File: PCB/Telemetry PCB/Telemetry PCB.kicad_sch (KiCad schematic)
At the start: 40 parts, among them IC1 E22-900M22S, J1 Conn_01x04_Pin, J2 GPS, J3 Batt, J4 Serial Debug Header 1x4, SW1 SW_MEC_5E, SW2 SW_MEC_5E, U1 STM32F411CEUx, U2 AP62200WU, U3 MCP1700x-250xxTT, Y1 25MHZ 9pF, Y2 32.768k 6pF

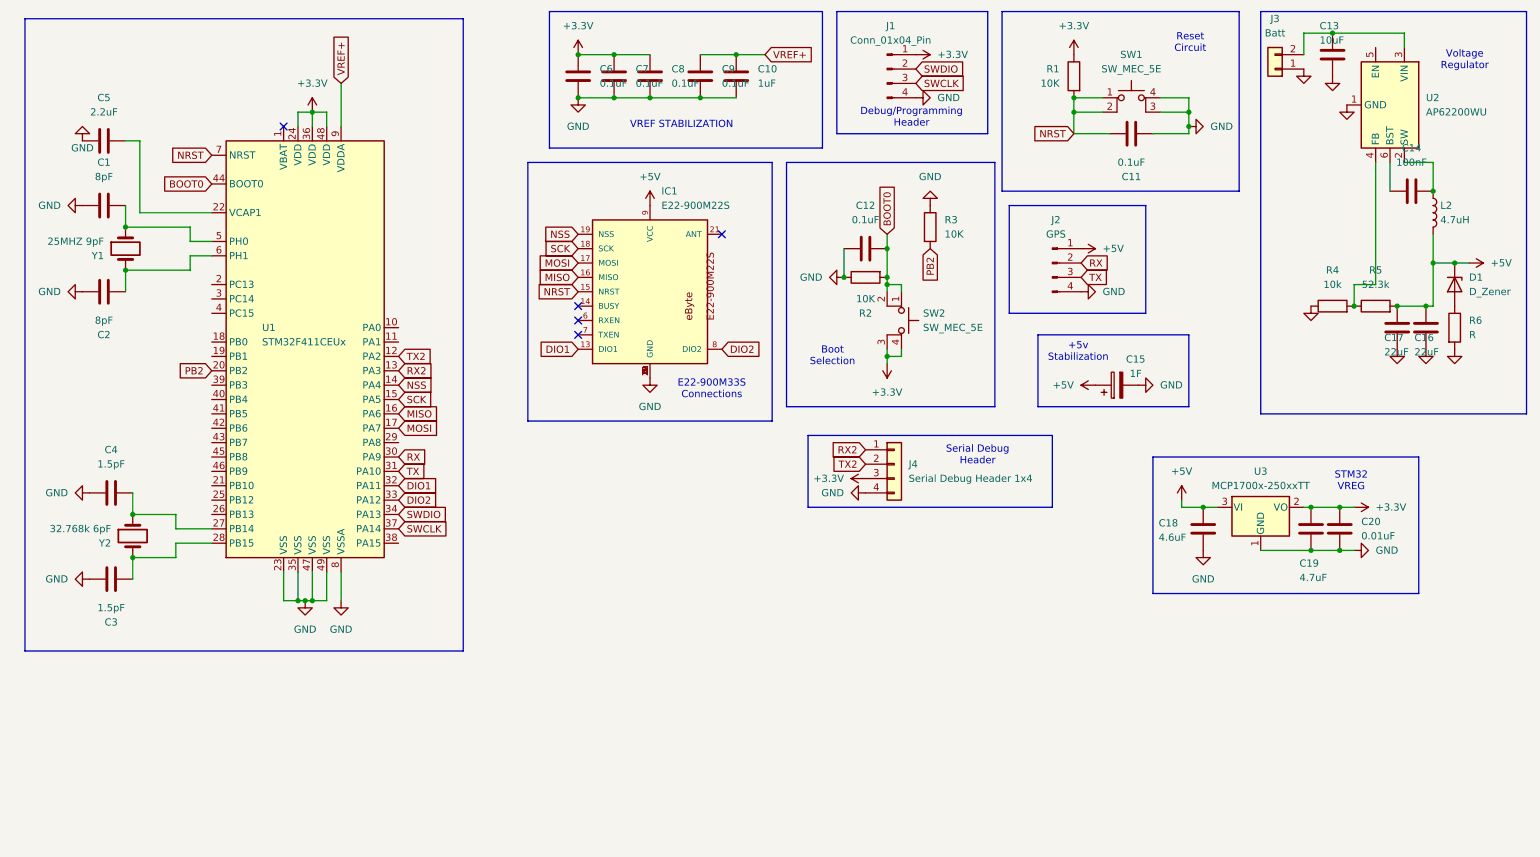
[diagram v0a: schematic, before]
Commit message: see last push discription
Last push did not work. see last push for description
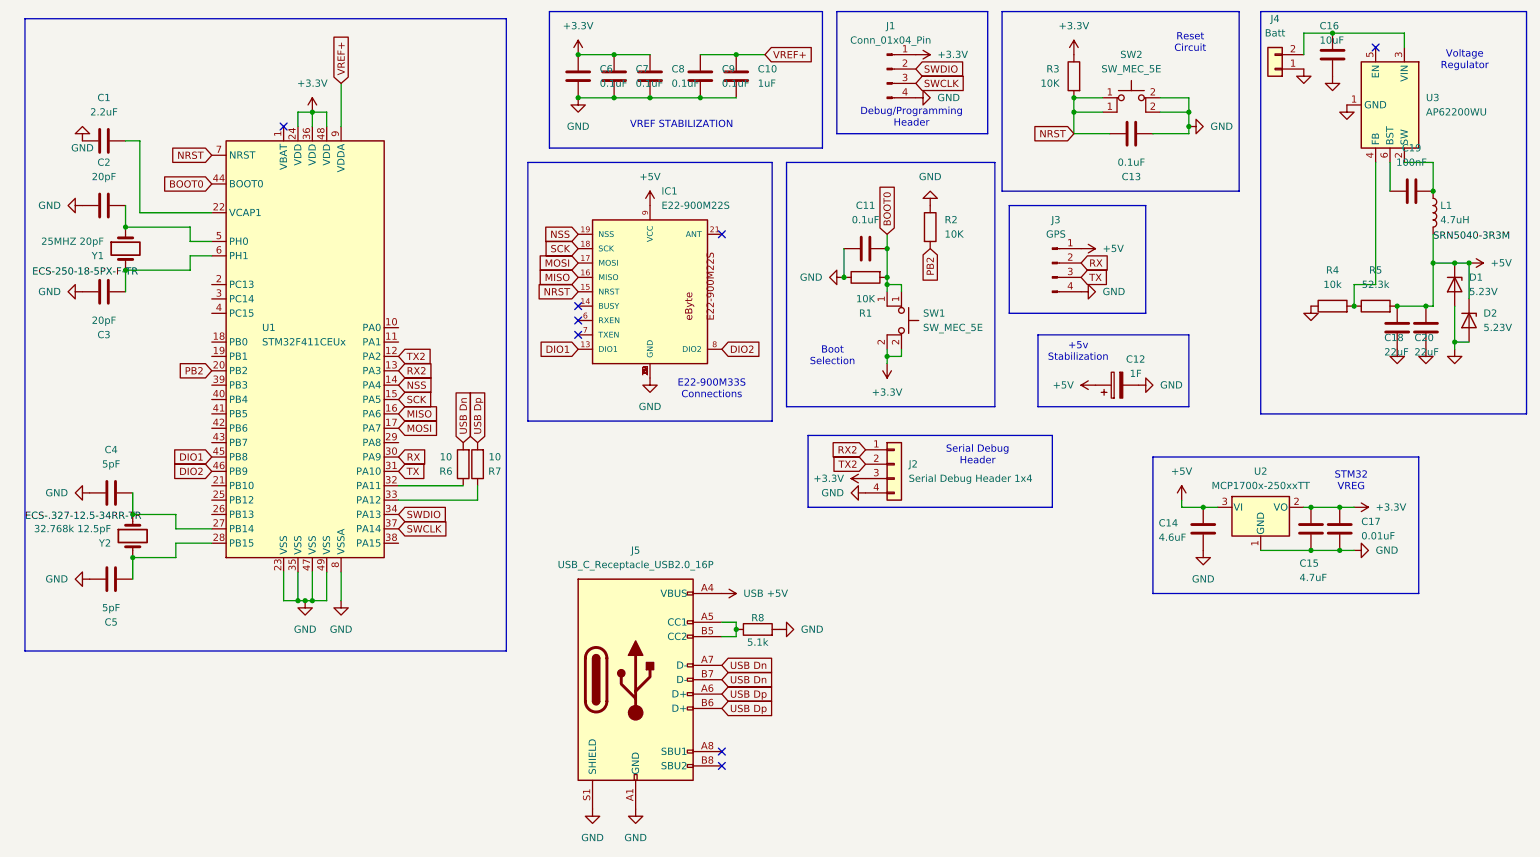
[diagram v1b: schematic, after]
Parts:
- removed SW1: SW_MEC_5E, Button_Switch_SMD:SW_Push_1P1T_NO_6x6mm_H9.5mm, symbol Switch:SW_MEC_5E
- added D2: 5.23V, PLZ5V1C_G3_H:CR_1C-G3&slash_H_VIS, symbol Device:D_Zener
- added J5: USB_C_Receptacle_USB2.0_16P, Connector_USB:USB_C_Receptacle_GCT_USB4105-xx-A_16P_TopMnt_Horizontal, symbol Connector:USB_C_Receptacle_USB2.0_16P
- added R7: 10, Capacitor_SMD:C_1206_3216Metric_Pad1.33x1.80mm_HandSolder, symbol Device:R
- added R8: 5.1k, Capacitor_SMD:C_1206_3216Metric_Pad1.33x1.80mm_HandSolder, symbol Device:R
- added SW2: SW_MEC_5E, Button_Switch_SMD:SW_Push_1P1T_NO_6x6mm_H9.5mm, symbol Switch:SW_MEC_5E
- C14: renamed from C18; footprint (none) -> Capacitor_SMD:C_1206_3216Metric_Pad1.33x1.80mm_HandSolder
- C15: renamed from C19; footprint (none) -> Capacitor_SMD:C_1206_3216Metric_Pad1.33x1.80mm_HandSolder
- C17: renamed from C20; footprint (none) -> Capacitor_SMD:C_1206_3216Metric_Pad1.33x1.80mm_HandSolder
- C2: renamed from C1; value 8pF -> 20pF
- C3: renamed from C2; value 8pF -> 20pF
- C4: value 1.5pF -> 5pF
- C5: renamed from C3; value 1.5pF -> 5pF
- D1: value D_Zener -> 5.23V; footprint (none) -> PLZ5V1C_G3_H:CR_1C-G3&slash_H_VIS
- L1: renamed from L2; footprint SRN5040TA-220M:SRN5040TA-220M -> SRN5040_3R3M:IND_SRN5040_BRN
- R6: value R -> 10; footprint Resistor_SMD:R_1206_3216Metric_Pad1.30x1.75mm_HandSolder -> Capacitor_SMD:C_1206_3216Metric_Pad1.33x1.80mm_HandSolder
- Y1: value 25MHZ 9pF -> 25MHZ 20pF; footprint (none) -> Crystal:Crystal_SMD_HC49-SD_HandSoldering
- Y2: value 32.768k 6pF -> 32.768k 12.5pF; footprint (none) -> ECS__327_12_5_34RR_TR:XTAL_ECS-.327-12.5-34RR-TR
- renumbered C5 to C1, C12 to C11, C15 to C12, C11 to C13, C13 to C16, C17 to C18, C14 to C19, C16 to C20, J4 to J2, J2 to J3, J3 to J4, R2 to R1, R3 to R2, R1 to R3, SW2 to SW1, U3 to U2, U2 to U3
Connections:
- net +3.3V: now also SW1.2 (K); no longer SW1.3 (K), SW1.4 (A)
- net +5V: now also D2.1 (K)
- net BOOT0: no longer SW1.2
- net DIO1: now also U1.45 (PB8); no longer U1.32 (PA11)
- net DIO2: now also U1.46 (PB9); no longer U1.33 (PA12)
- net GND: now also D1.2 (A), D2.2 (A), J5.A1 (GND), J5.A12 (GND), J5.B1 (GND), J5.B12 (GND), J5.S1 (SHIELD), R8.2, SW2.2 (K); no longer R6.2
- net NRST: now also SW2.1
- net at R6.1: now also U1.32 (PA11); no longer D1.2 (A)
- new net: R7.1, U1.33 (PA12)
- new net: J5.A5 (CC1), J5.B5 (CC2), R8.1
- new net USB +5V: J5.A4 (VBUS), J5.A9 (VBUS), J5.B4 (VBUS), J5.B9 (VBUS)
- new net USB Dn: J5.A7 (D-), J5.B7 (D-), R6.2
- new net USB Dp: J5.A6 (D+), J5.B6 (D+), R7.2
- no-connect marks 5 -> 8
